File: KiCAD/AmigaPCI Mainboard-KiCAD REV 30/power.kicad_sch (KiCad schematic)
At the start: 82 parts, among them CN205 POW SW, CN206 RESET, CN600 Conn_01x03_Pin, CN601 ATX-24, J1 _TA, J10 _RESET, J11 _REGEN, J12 _TBI, J2 CLK7, J210 Case Fan, J5 _TS, J6 _TIP, J7 TT0, J8 TT1, U206 DS1818R-10+T&R, U215 74HCT03, U219 74AHCT04, U220 74LVC08, U222 74HCT4066, U229 74CBT16233, U303 74HCT74, U600 STM8S001J3M, U601 AP2114H-1.2, U818 74AHC1G09

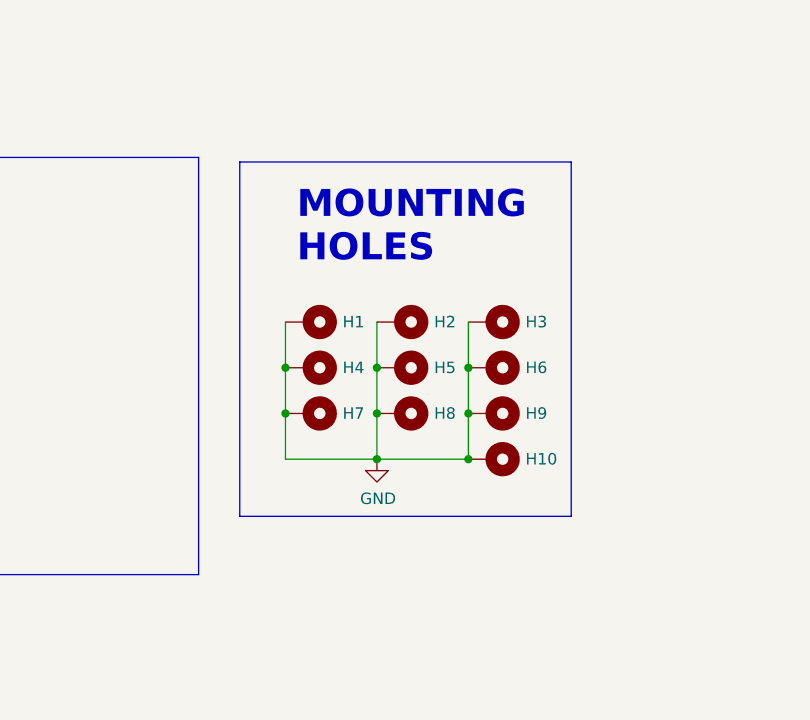
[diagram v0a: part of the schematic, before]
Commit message: Rev 3.0 PCB Routing 12-MAY-2024
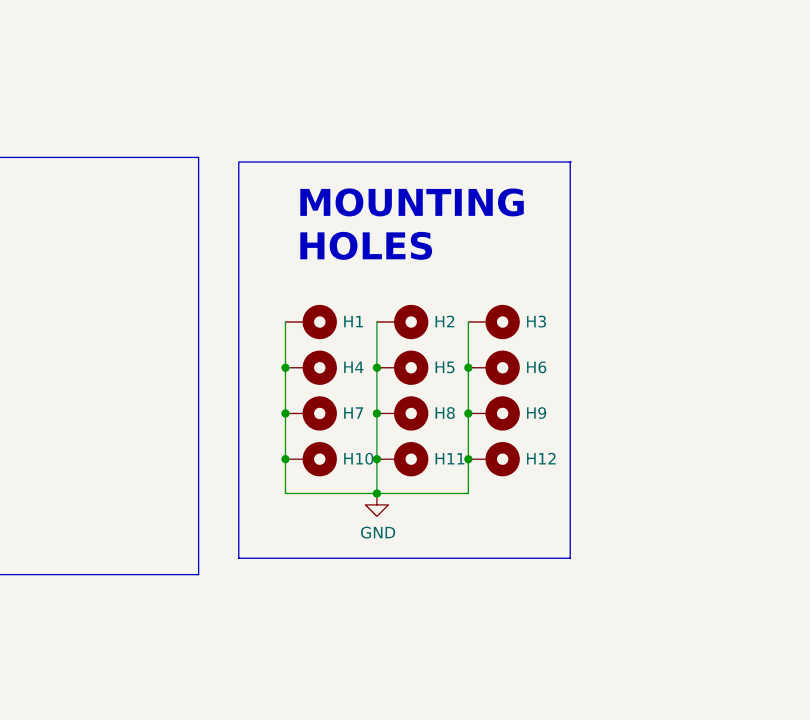
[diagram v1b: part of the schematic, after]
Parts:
- added H11, H12: MountingHole_Pad, MountingHole:MountingHole_2.2mm_M2_DIN965_Pad, symbol Mechanical:MountingHole_Pad
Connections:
- net GND: now also H11.1, H12.1
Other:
- moved on the sheet: H10
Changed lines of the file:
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@@
 	)
 	(junction
+		(at 337.82 177.8)
+		(diameter 0)
+		(color 0 0 0 0)
+	)
+	(junction
 		(at 66.04 176.53)
 		(diameter 0)
@@
 	)
 	(junction
-		(at 347.98 173.99)
-		(diameter 0)
-		(color 0 0 0 0)
-	)
-	(junction
 		(at 140.97 95.25)
 		(diameter 0)
@@
 	)
 	(junction
+		(at 337.82 173.99)
+		(diameter 0)
+		(color 0 0 0 0)
+	)
+	(junction
 		(at 92.71 39.37)
 		(diameter 0)
@@
 	)
 	(junction
+		(at 347.98 173.99)
+		(diameter 0)
+		(color 0 0 0 0)
+	)
+	(junction
 		(at 111.76 55.88)
 		(diameter 0)
@@
 	)
 	(junction
-		(at 86.36 156.21)
+		(at 327.66 173.99)
 		(diameter 0)
 		(color 0 0 0 0)
 	)
 	(junction
-		(at 204.47 204.47)
+		(at 86.36 156.21)
 		(diameter 0)
 		(color 0 0 0 0)
 	)
 	(junction
-		(at 337.82 163.83)
+		(at 204.47 204.47)
 		(diameter 0)
 		(color 0 0 0 0)
 	)
 	(junction
-		(at 337.82 173.99)
+		(at 337.82 163.83)
 		(diameter 0)
 		(color 0 0 0 0)
@@
 	(polyline
 		(pts
-			(xy 322.58 180.34) (xy 359.41 180.34)
+			(xy 322.47 185) (xy 359.3 185)
 		)
 		(stroke
@@
 	(wire
 		(pts
-			(xy 86.36 161.29) (xy 86.36 156.21)
+			(xy 347.98 173.99) (xy 347.98 177.8)
 		)
 		(stroke
@@
 	(wire
 		(pts
-			(xy 337.82 168.91) (xy 337.82 173.99)
+			(xy 86.36 161.29) (xy 86.36 156.21)
 		)
 		(stroke
@@
 	(wire
 		(pts
-			(xy 347.98 173.99) (xy 347.98 168.91)
-		)
-		(stroke
-			(width 0)
-			(type default)
-		)
-	)
-	(wire
-		(pts
 			(xy 83.82 204.47) (xy 97.79 204.47)
 		)
@@
 	(wire
 		(pts
+			(xy 327.66 173.99) (xy 327.66 177.8)
+		)
+		(stroke
+			(width 0)
+			(type default)
+		)
+	)
+	(wire
+		(pts
 			(xy 92.71 50.8) (xy 104.14 50.8)
 		)
@@
 	(polyline
 		(pts
-			(xy 322.58 140.97) (xy 322.58 180.34)
+			(xy 322.47 140.97) (xy 322.47 185)
 		)
 		(stroke
@@
 	(wire
 		(pts
-			(xy 327.66 173.99) (xy 337.82 173.99)
+			(xy 327.66 177.8) (xy 337.82 177.8)
 		)
 		(stroke
@@
 	(wire
 		(pts
+			(xy 337.82 173.99) (xy 337.82 177.8)
+		)
+		(stroke
+			(width 0)
+			(type default)
+		)
+	)
+	(wire
+		(pts
 			(xy 132.08 44.45) (xy 140.97 44.45)
 		)
@@
 	(wire
 		(pts
+			(xy 337.82 168.91) (xy 337.82 173.99)
+		)
+		(stroke
+			(width 0)
+			(type default)
+		)
+	)
+	(wire
+		(pts
 			(xy 31.75 39.37) (xy 34.29 39.37)
 		)
@@
 	(wire
 		(pts
+			(xy 347.98 168.91) (xy 347.98 173.99)
+		)
+		(stroke
+			(width 0)
+			(type default)
+		)
+	)
+	(wire
+		(pts
 			(xy 86.36 161.29) (xy 88.9 161.29)
 		)
@@
 	(polyline
 		(pts
-			(xy 359.41 180.34) (xy 359.41 140.97)
+			(xy 359.3 185) (xy 359.3 140.97)
 		)
 		(stroke
@@
 	(wire
 		(pts
-			(xy 337.82 173.99) (xy 347.98 173.99)
+			(xy 337.82 177.8) (xy 347.98 177.8)
 		)
 		(stroke
@@
 	)
 	(symbol
+		(lib_id "Mechanical:MountingHole_Pad")
+		(at 350.52 173.99 270)
+		(unit 1)
+		(exclude_from_sim no)
+		(in_bom no)
+		(on_board yes)
+		(dnp no)
+		(property "Reference" "H12"
+			(at 354.33 173.99 90)
+			(effects
+				(font
+					(size 1.27 1.27)
+				)
+				(justify left)
+			)
+		)
+		(property "Value" "MountingHole_Pad"
+			(at 354.33 175.133 90)
+			(effects
+				(font
+					(size 1.27 1.27)
+				)
+				(justify left)
+				(hide yes)
+			)
+		)
+		(property "Footprint" "MountingHole:MountingHole_2.2mm_M2_DIN965_Pad"
+			(at 350.52 173.99 0)
+			(effects
+				(font
+					(size 1.27 1.27)
+				)
+				(hide yes)
+			)
+		)
+		(property "Datasheet" "~"
+			(at 350.52 173.99 0)
+			(effects
+				(font
+					(size 1.27 1.27)
+				)
+				(hide yes)
+			)
+		)
+		(property "Description" ""
+			(at 350.52 173.99 0)
+			(effects
+				(font
+					(size 1.27 1.27)
+				)
+				(hide yes)
+			)
+		)
+		(pin "1"
+		)
+		(instances
+			(project "AmigaPCI Mainboard"
+				(path "/72453515-27fe-4336-91f3-e3c8054f7767/4cb777ef-2899-49f4-b38f-a0c07d84fa7d"
+					(reference "H12")
+					(unit 1)
+				)
+			)
+		)
+	)
+	(symbol
 		(lib_id "Device:R_Small")
 		(at 128.27 105.41 90)
@@
 	(symbol
 		(lib_id "power:GND")
-		(at 337.82 173.99 0)
+		(at 337.82 177.8 0)
 		(unit 1)
 		(exclude_from_sim no)
@@
 		(dnp no)
 		(property "Reference" "#PWR0357"
-			(at 337.82 180.34 0)
+			(at 337.82 184.15 0)
 			(effects
 				(font
@@
 		)
 		(property "Value" "GND"
-			(at 337.947 178.3842 0)
+			(at 337.947 182.1942 0)
 			(effects
 				(font
@@
 		)
 		(property "Footprint" ""
-			(at 337.82 173.99 0)
+			(at 337.82 177.8 0)
 			(effects
 				(font
@@
 		)
 		(property "Datasheet" ""
-			(at 337.82 173.99 0)
+			(at 337.82 177.8 0)
 			(effects
 				(font
@@
 		)
 		(property "Description" ""
-			(at 337.82 173.99 0)
+			(at 337.82 177.8 0)
 			(effects
 				(font
@@
 	)
 	(symbol
+		(lib_id "Mechanical:MountingHole_Pad")
+		(at 340.36 173.99 270)
+		(unit 1)
+		(exclude_from_sim no)
+		(in_bom no)
+		(on_board yes)
+		(dnp no)
+		(property "Reference" "H11"
+			(at 344.17 173.99 90)
+			(effects
+				(font
+					(size 1.27 1.27)
+				)
+				(justify left)
+			)
+		)
+		(property "Value" "MountingHole_Pad"
+			(at 344.17 175.133 90)
+			(effects
+				(font
+					(size 1.27 1.27)
+				)
+				(justify left)
+				(hide yes)
+			)
+		)
+		(property "Footprint" "MountingHole:MountingHole_2.2mm_M2_DIN965_Pad"
+			(at 340.36 173.99 0)
+			(effects
+				(font
+					(size 1.27 1.27)
+				)
+				(hide yes)
+			)
+		)
+		(property "Datasheet" "~"
+			(at 340.36 173.99 0)
+			(effects
+				(font
+					(size 1.27 1.27)
+				)
+				(hide yes)
+			)
+		)
+		(property "Description" ""
+			(at 340.36 173.99 0)
+			(effects
+				(font
+					(size 1.27 1.27)
+				)
+				(hide yes)
+			)
+		)
+		(pin "1"
+		)
+		(instances
+			(project "AmigaPCI Mainboard"
+				(path "/72453515-27fe-4336-91f3-e3c8054f7767/4cb777ef-2899-49f4-b38f-a0c07d84fa7d"
+					(reference "H11")
+					(unit 1)
+				)
+			)
+		)
+	)
+	(symbol
 		(lib_id "power:+3V3")
 		(at 121.92 91.44 0)
@@
 	(symbol
 		(lib_id "Mechanical:MountingHole_Pad")
-		(at 350.52 173.99 270)
+		(at 330.2 173.99 270)
 		(unit 1)
 		(exclude_from_sim no)
@@
 		(dnp no)
 		(property "Reference" "H10"
-			(at 354.33 173.99 90)
+			(at 334.01 173.99 90)
 			(effects
 				(font
@@
 		)
 		(property "Value" "MountingHole_Pad"
-			(at 354.33 175.133 90)
+			(at 334.01 175.133 90)
 			(effects
 				(font
@@
 		)
 		(property "Footprint" "MountingHole:MountingHole_4mm_Pad_Via"
-			(at 350.52 173.99 0)
+			(at 330.2 173.99 0)
 			(effects
 				(font
@@
 		)
 		(property "Datasheet" "~"
-			(at 350.52 173.99 0)
+			(at 330.2 173.99 0)
 			(effects
 				(font
@@
 		)
 		(property "Description" ""
-			(at 350.52 173.99 0)
+			(at 330.2 173.99 0)
 			(effects
 				(font
